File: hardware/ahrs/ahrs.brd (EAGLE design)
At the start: 30 x 30 mm, 32 parts, among them J1 2-PIN, U1 LSM9DS1, U2 STM32G4_UFQFPN48_T1, X1 NX2016SA24MHZ-EXS00A-CS11335, X2 SM08B-SRSS-TB

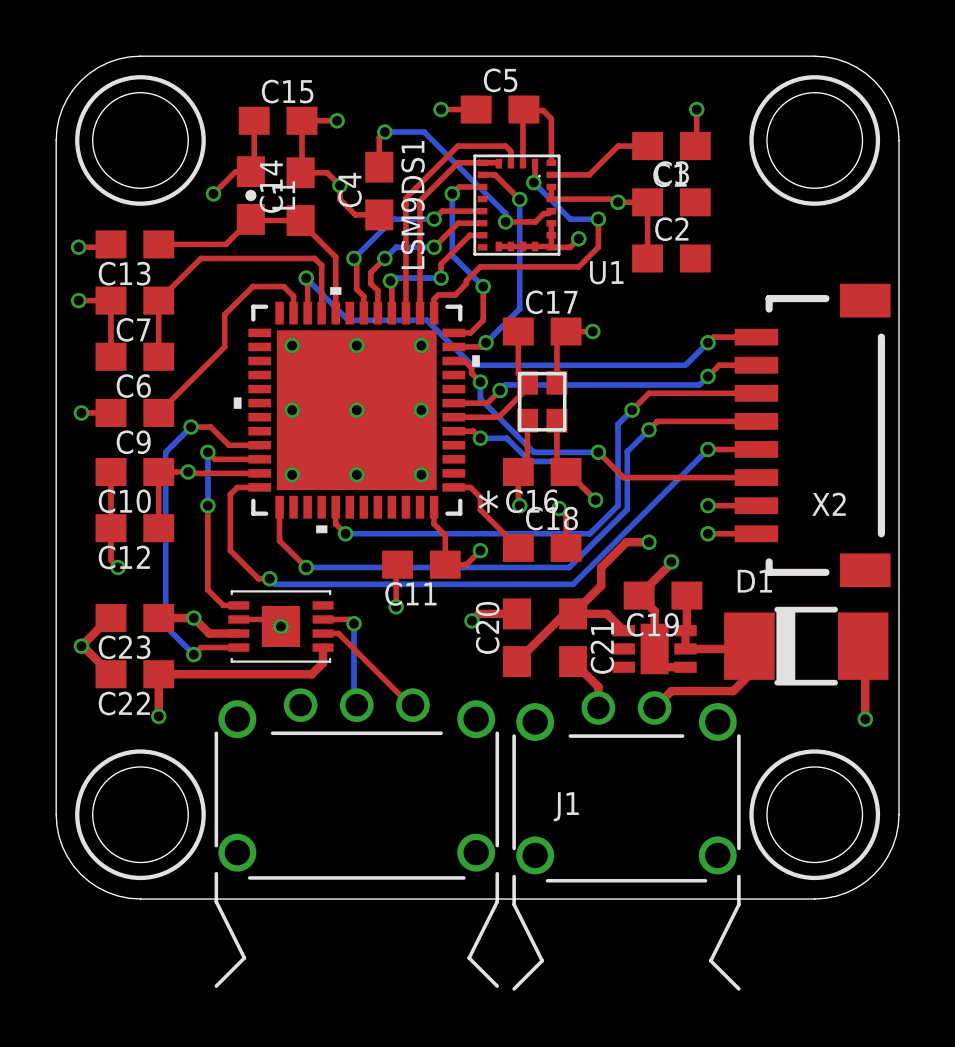
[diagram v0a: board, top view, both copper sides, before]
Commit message: Rerouting much better
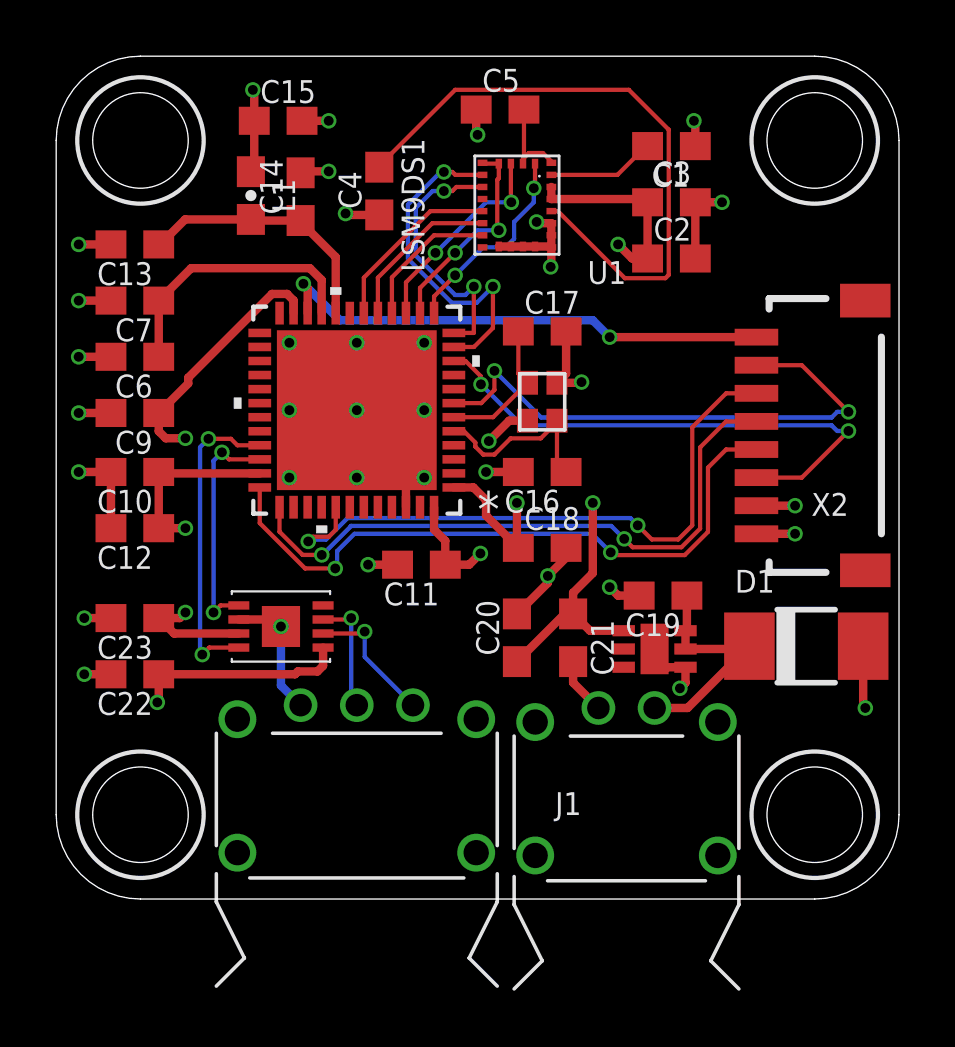
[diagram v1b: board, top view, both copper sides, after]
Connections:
- net N$1 renamed VDDA
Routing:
- net N$3: track 8.92 -> 22.4 mm, vias 2 -> 0
- net NRST: track 11.3 -> 19.7 mm
- net LPUART_TX: track 12.9 -> 19.2 mm
- net SCK: track 11.7 -> 7.28 mm
- net CS_AG: track 8.49 -> 12.2 mm
- net SWO: track 19.5 -> 22.8 mm
- net 3.3V: track 50.2 -> 53.3 mm, vias 8 -> 10
- net N$6: track 9.48 -> 6.59 mm, vias 2 -> 0
- net CS_M: track 7.36 -> 9.51 mm
- net CAN_RX: track 13.3 -> 11.2 mm
- net MOSI: track 9.11 -> 7.41 mm, vias 0 -> 2
- net N$4: track 4.64 -> 3.38 mm
- net LPUART_RX: track 19.0 -> 18.0 mm
- net INT_M: track 7.36 -> 6.47 mm, vias 2 -> 0
- net GND: track 48.0 -> 48.7 mm, vias 27 -> 33
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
